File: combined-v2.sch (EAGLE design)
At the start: 385 parts, among them IC2 PCM1865DBT, U11 TMUX1204DGSR, U2 LM4562MAX/NOPB, U3 TMUX1204DGSR, U4 TMUX1204DGSR, U5 TMUX1204DGSR, Y2 ECS-245.7-20-3X-EN-TR

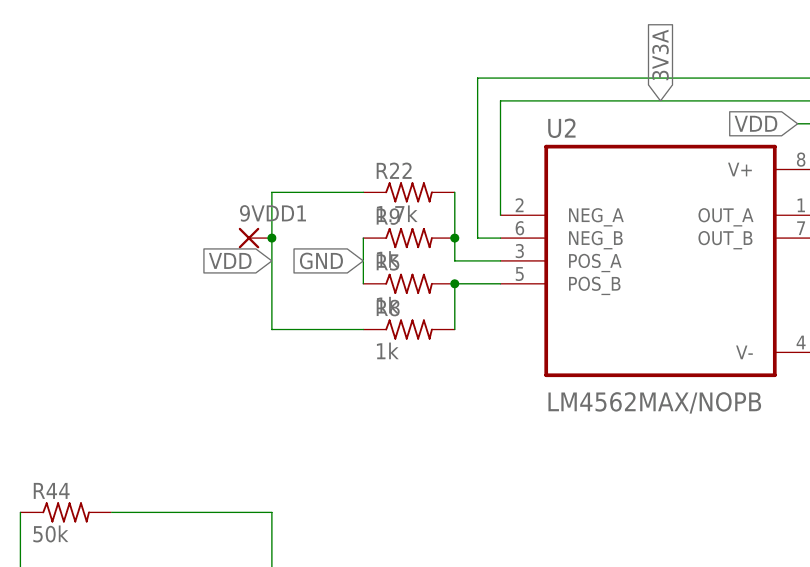
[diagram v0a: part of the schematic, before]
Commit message: update power resisitors
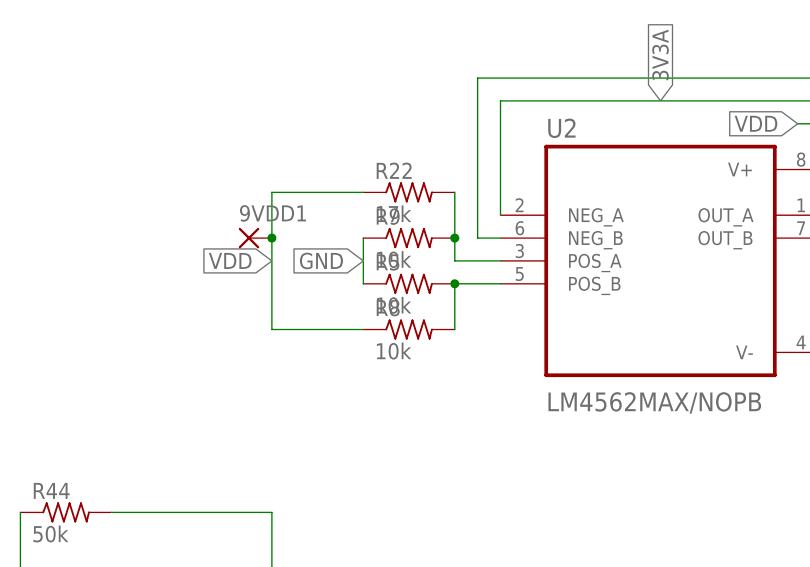
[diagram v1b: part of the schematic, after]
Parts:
- R22: value 1.7k -> 17k
- R5, R8, R9: value 1k -> 10k
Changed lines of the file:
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@@
 <part name="R166" library="rcl" library_urn="urn:adsk.eagle:library:334" deviceset="R-US_" device="R0402" package3d_urn="urn:adsk.eagle:package:23547/3" value="100k"/>
 <part name="U2" library="LM4562MAX_NOPB" deviceset="LM4562MAX/NOPB" device=""/>
-<part name="R5" library="rcl" library_urn="urn:adsk.eagle:library:334" deviceset="R-US_" device="R0402" package3d_urn="urn:adsk.eagle:package:23547/3" value="1k"/>
-<part name="R8" library="rcl" library_urn="urn:adsk.eagle:library:334" deviceset="R-US_" device="R0402" package3d_urn="urn:adsk.eagle:package:23547/3" value="1k"/>
-<part name="R9" library="rcl" library_urn="urn:adsk.eagle:library:334" deviceset="R-US_" device="R0402" package3d_urn="urn:adsk.eagle:package:23547/3" value="1k"/>
-<part name="R22" library="rcl" library_urn="urn:adsk.eagle:library:334" deviceset="R-US_" device="R0402" package3d_urn="urn:adsk.eagle:package:23547/3" value="1.7k"/>
+<part name="R5" library="rcl" library_urn="urn:adsk.eagle:library:334" deviceset="R-US_" device="R0402" package3d_urn="urn:adsk.eagle:package:23547/3" value="10k"/>
+<part name="R8" library="rcl" library_urn="urn:adsk.eagle:library:334" deviceset="R-US_" device="R0402" package3d_urn="urn:adsk.eagle:package:23547/3" value="10k"/>
+<part name="R9" library="rcl" library_urn="urn:adsk.eagle:library:334" deviceset="R-US_" device="R0402" package3d_urn="urn:adsk.eagle:package:23547/3" value="10k"/>
+<part name="R22" library="rcl" library_urn="urn:adsk.eagle:library:334" deviceset="R-US_" device="R0402" package3d_urn="urn:adsk.eagle:package:23547/3" value="17k"/>
 <part name="9VDD1" library="wirepad" library_urn="urn:adsk.eagle:library:412" deviceset="SMD2" device="" package3d_urn="urn:adsk.eagle:package:30839/1"/>
 <part name="GND4" library="wirepad" library_urn="urn:adsk.eagle:library:412" deviceset="SMD2" device="" package3d_urn="urn:adsk.eagle:package:30839/1"/>

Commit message: replace incorrect diode size
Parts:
- D16, D17, D18, D19, D2, D20, D21, D22, D23, D24, D25, D26, D27, D28, D29, D3, D30, D31, D32, D33, D34, D35, D36, D37, D38, D39, D4, D40, D41, D42, D43, D44, D45, D46, D47, D48, D5, D60, D61, D62, D63, D64, D65, D66, D67, D68, D69, D70: device 1N4148W-TP:1N4148W-TP -> 1N4148W-TP(1):1N4148W-TP
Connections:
- net L1_COMP1: now also D19.1; no longer D19.C
- net L1_COMP2: now also D41.1; no longer D41.C
- net L1_COMP3: now also D30.1; no longer D30.C
- net L1_COMP4: now also D63.1; no longer D63.C
- net N$100: now also D64.2, D65.1; no longer D64.A, D65.C
- net N$102: now also D68.2, D69.1; no longer D68.A, D69.C
- net N$103: now also D67.2, D68.1; no longer D67.A, D68.C
- net N$211: now also D17.2, D18.1, D25.2; no longer D17.A, D18.C, D25.A
- net N$212: now also D39.2, D40.1, D47.2; no longer D39.A, D40.C, D47.A
- net N$213: now also D28.2, D29.1, D36.2; no longer D28.A, D29.C, D36.A
- net N$214: now also D61.2, D62.1, D69.2; no longer D61.A, D62.C, D69.A
- net N$74: now also D16.2, D17.1; no longer D16.A, D17.C
- net N$75: now also D21.2, D22.1; no longer D21.A, D22.C
- net N$76: now also D20.2, D21.1; no longer D20.A, D21.C
- net N$78: now also D24.2, D25.1; no longer D24.A, D25.C
- net N$79: now also D23.2, D24.1; no longer D23.A, D24.C
- net N$80: now also D27.2, D28.1; no longer D27.A, D28.C
- net N$81: now also D32.2, D33.1; no longer D32.A, D33.C
- net N$82: now also D31.2, D32.1; no longer D31.A, D32.C
- net N$84: now also D35.2, D36.1; no longer D35.A, D36.C
- net N$85: now also D34.2, D35.1; no longer D34.A, D35.C
- net N$86: now also D38.2, D39.1; no longer D38.A, D39.C
- net N$87: now also D43.2, D44.1; no longer D43.A, D44.C
- net N$88: now also D42.2, D43.1; no longer D42.A, D43.C
- net N$90: now also D46.2, D47.1; no longer D46.A, D47.C
- net N$91: now also D45.2, D46.1; no longer D45.A, D46.C
- net N$98: now also D60.2, D61.1; no longer D60.A, D61.C
- net N$99: now also D65.2, D66.1; no longer D65.A, D66.C
- net NEG_A1_COMP1: now also D16.1, D18.2; no longer D16.C, D18.A
- net NEG_A1_COMP2: now also D38.1, D40.2; no longer D38.C, D40.A
- net NEG_A1_COMP3: now also D27.1, D29.2; no longer D27.C, D29.A
- net NEG_A1_COMP4: now also D60.1, D62.2; no longer D60.C, D62.A
- net OUT_A3_COMP1: now also D26.2; no longer D26.A
- net OUT_A3_COMP2: now also D48.2; no longer D48.A
- net OUT_A3_COMP3: now also D37.2; no longer D37.A
- net OUT_A3_COMP4: now also D70.2; no longer D70.A
- net OUT_B1_COMP1: now also D19.2; no longer D19.A
- net OUT_B1_COMP2: now also D41.2; no longer D41.A
- net OUT_B1_COMP3: now also D30.2; no longer D30.A
- net OUT_B1_COMP4: now also D63.2; no longer D63.A
- net OUT_B3_COMP1: now also D20.1; no longer D20.C
- net OUT_B3_COMP2: now also D42.1; no longer D42.C
- net OUT_B3_COMP3: now also D31.1; no longer D31.C
- net OUT_B3_COMP4: now also D64.1; no longer D64.C
- net P0W_PAN1: now also D2.1; no longer D2.C
- net P0W_PAN2: now also D4.1; no longer D4.C
- net P0W_PAN3: now also D3.1; no longer D3.C
- net P0W_PAN4: now also D5.1; no longer D5.C
- net POS_A4_COMP1: now also D22.2, D23.1; no longer D22.A, D23.C
- net POS_A4_COMP2: now also D44.2, D45.1; no longer D44.A, D45.C
- net POS_A4_COMP3: now also D33.2, D34.1; no longer D33.A, D34.C
- net POS_A4_COMP4: now also D66.2, D67.1; no longer D66.A, D67.C
- net POS_B1_COMP1: now also D26.1; no longer D26.C
- net POS_B1_COMP2: now also D48.1; no longer D48.C
- net POS_B1_COMP3: now also D37.1; no longer D37.C
- net POS_B1_COMP4: now also D70.1; no longer D70.C
- net VREF: now also D2.2, D3.2, D4.2, D5.2; no longer D2.A, D3.A, D4.A, D5.A
